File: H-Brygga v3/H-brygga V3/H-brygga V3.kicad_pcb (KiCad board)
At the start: 2 copper layers, 78.2 x 63.2 mm, 33 parts, among them J1 POWER, J2 sensor vänster, J3 SERVO, J4 sensor motor, J5 START, J6 sensor höger, J7 MOTOR, J8 Högtalare, P1 Digital, P2 Analog, P7 Digital, P8 Analog, SW1 SW_MEC_5E, SW2 SW_MEC_5E, U1 L298HN, U2 DFR0299

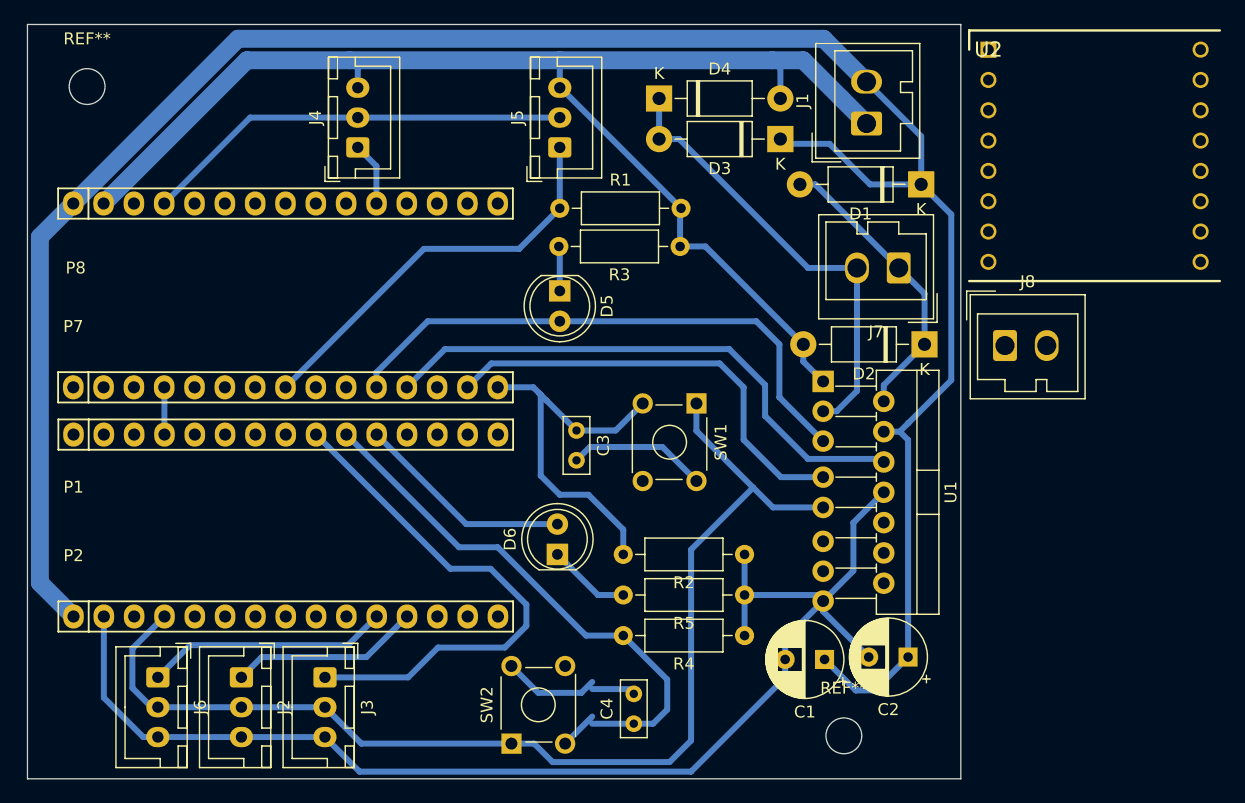
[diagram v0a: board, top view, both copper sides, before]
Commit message: H-brygga inför fräsning
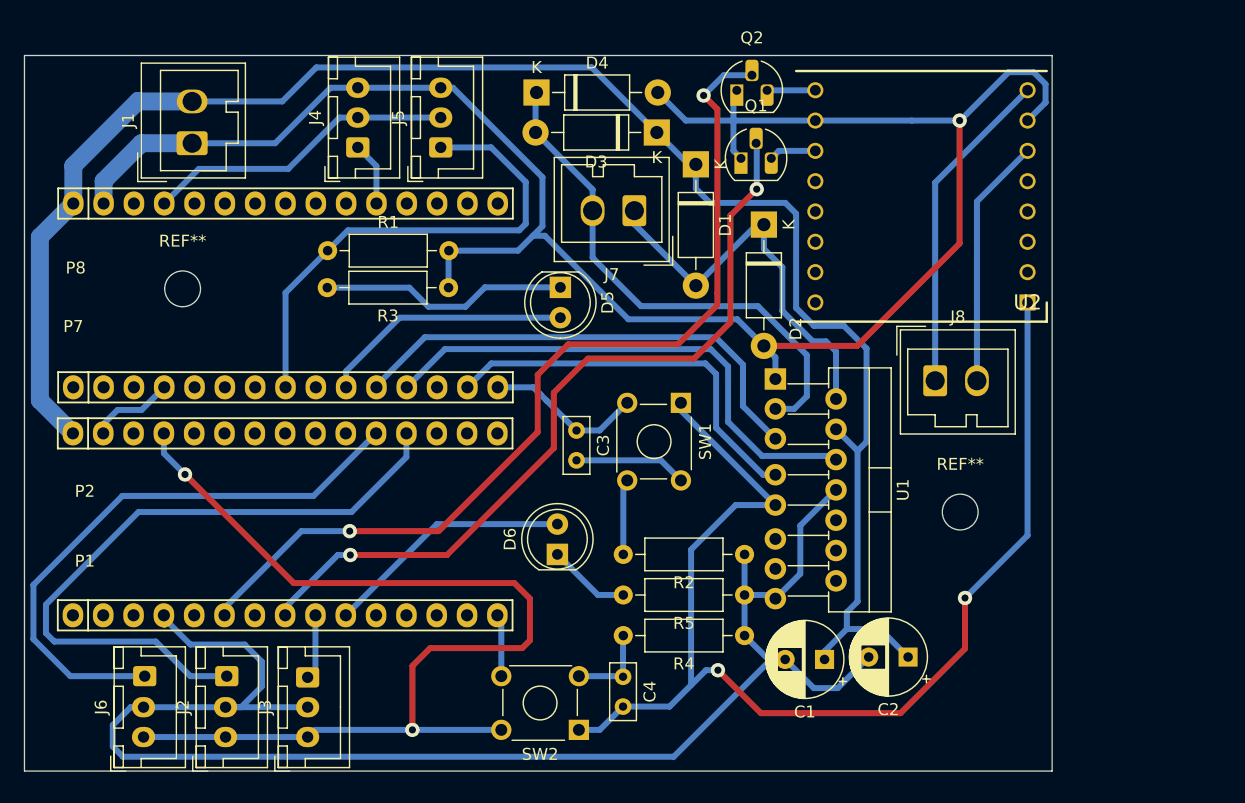
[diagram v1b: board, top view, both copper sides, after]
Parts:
- added Q1: Q_NMOS_DGS, Package_TO_SOT_THT:TO-92_HandSolder, F.Cu at (77.6, 88.4)
- added Q2: Q_NMOS_DGS, Package_TO_SOT_THT:TO-92_HandSolder, F.Cu at (77.2, 82.7)
- U2: footprint footprints:DIPS1778W50P254L2100H170Q16N -> Egna:DIPS1778W50P254L2100H170Q16N
- moved J1 56.5 mm to (31.6, 87.2)
- moved J7 22.7 mm to (68.7, 92.8)
- moved U2 21.4 mm to (101.6, 100.5), turned to 180 degrees
- moved REF** 21.1 mm to (96.0, 118.0)
- moved R1 19.8 mm to (43.0, 96.2)
- moved R3 19.7 mm to (53.1, 99.2)
- moved D1 19.0 mm to (73.8, 88.9), turned to -90 degrees
- moved REF** 18.7 mm to (30.8, 99.3)
- moved D2 16.8 mm to (79.5, 94.0), turned to -90 degrees
- moved P2 15.3 mm to (21.6, 111.5)
- moved P1 15.1 mm to (21.6, 126.7)
- moved D3 10.4 mm to (70.5, 86.2)
- moved D4 10.3 mm to (60.5, 82.9)
- moved J5 9.98 mm to (52.4, 87.5)
- moved J8 6.55 mm to (93.8, 107.0)
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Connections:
- C3 pad 2: Net-(C3-Pad2) -> MP3+
- C4 pad 1: 7. -> 12(MISO).
- C4 pad 2: Net-(C4-Pad2) -> MP3+
- D5 pad 2: 8a -> 7a
- D6 pad 2: 8. -> 7.
- J2 pad 2: +5V -> MP3+
- J3 pad 2: +5V -> MP3+
- J4 pad 2: +5V -> MP3+
- J5 pad 2: +5V -> MP3+
- J6 pad 2: +5V -> MP3+
- P1 pad 11: 8. -> /8.
- P1 pad 15: /12(MISO). -> 12(MISO).
- P1 pad 6: /3(**). -> 3(**).
- P1 pad 8: /5(**). -> 5(**).
- P2 pad 4: +5V -> MP3+
- P7 pad 10: /7a -> 7a
- P8 pad 4: +5V -> MP3+
- R4 pad 2: 7. -> 12(MISO).
- SW1 pad 1: +5V -> MP3+
- SW1 pad 2: Net-(C3-Pad2) -> MP3+
- SW1 pad 4: unconnected-(SW1-Pad4) -> 12(MISO)
- SW2 pad 1: +5V -> MP3+
- SW2 pad 2: Net-(C4-Pad2) -> MP3+
- SW2 pad 3: 7. -> 12(MISO).
- SW2 pad 4: unconnected-(SW2-Pad4) -> 12(MISO).
- U1 pad 9: +5V -> MP3+
- U2 pad 11: Next -> Net-(U2-Pad11)
- U2 pad 9: Previous -> Net-(U2-Pad9)
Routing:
- net MP3+: track 0.00 -> 223.9 mm, vias 0 -> 4
- net +5V: track 132.6 -> 0.00 mm
- net 3(**).: track 0.00 -> 78.0 mm, vias 0 -> 2
- net GND: track 227.2 -> 299.1 mm, vias 0 -> 1
- net 5(**).: track 0.00 -> 66.5 mm, vias 0 -> 2
- net Vin: track 188.0 -> 146.4 mm
- net A0.: track 16.0 -> 56.3 mm
- net 6(**).: track 44.0 -> 5.47 mm
- net A1.: track 20.4 -> 49.1 mm
- net Net-(J8-Pad1): track 0.00 -> 27.5 mm
- net 7.: track 47.9 -> 20.9 mm
- net 7a: track 0.00 -> 21.2 mm
- net Net-(J8-Pad2): track 0.00 -> 21.0 mm
- net 8.: track 18.2 -> 0.00 mm
- net Net-(D5-Pad1): track 3.76 -> 20.9 mm
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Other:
- board size 78.2 x 63.2 mm -> 86.1 x 60 mm
